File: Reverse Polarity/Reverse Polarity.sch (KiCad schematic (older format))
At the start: 16 parts, among them P1 CONN_01X04, P2 CONN_01X04, P3 CONN_01X04, P4 CONN_01X04, P5 CONN_01X04, P6 CONN_01X04, P7 CONN_01X04, P8 CONN_01X04

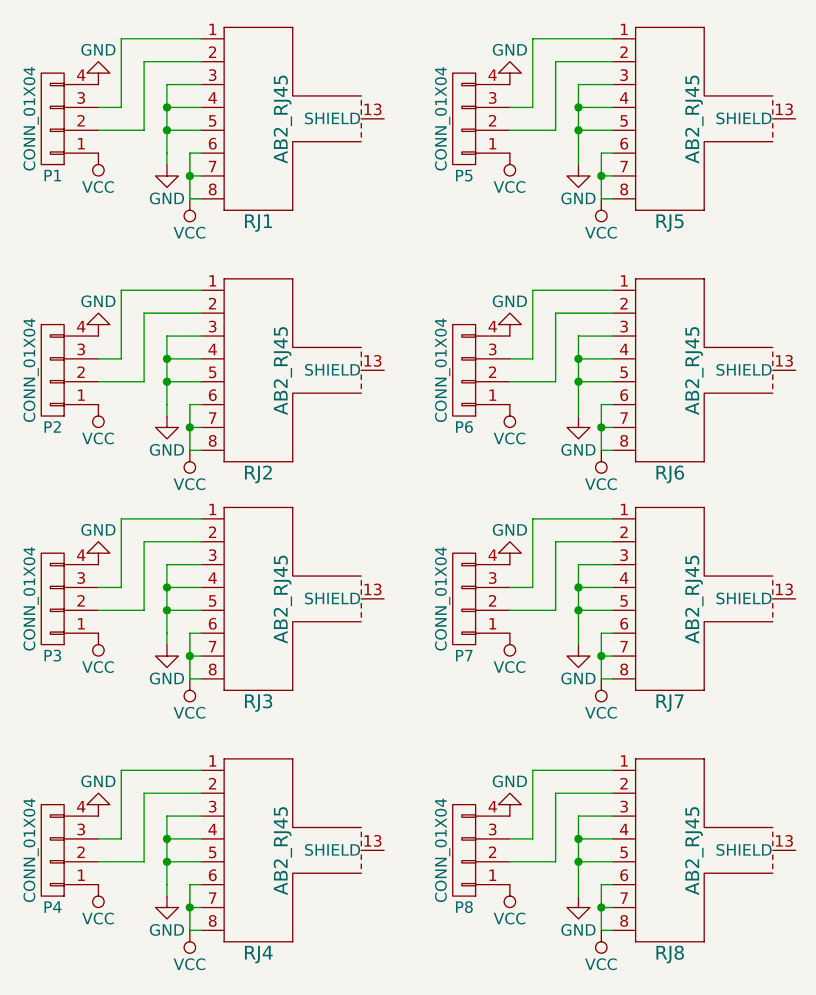
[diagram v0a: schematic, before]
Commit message: Also update schematic
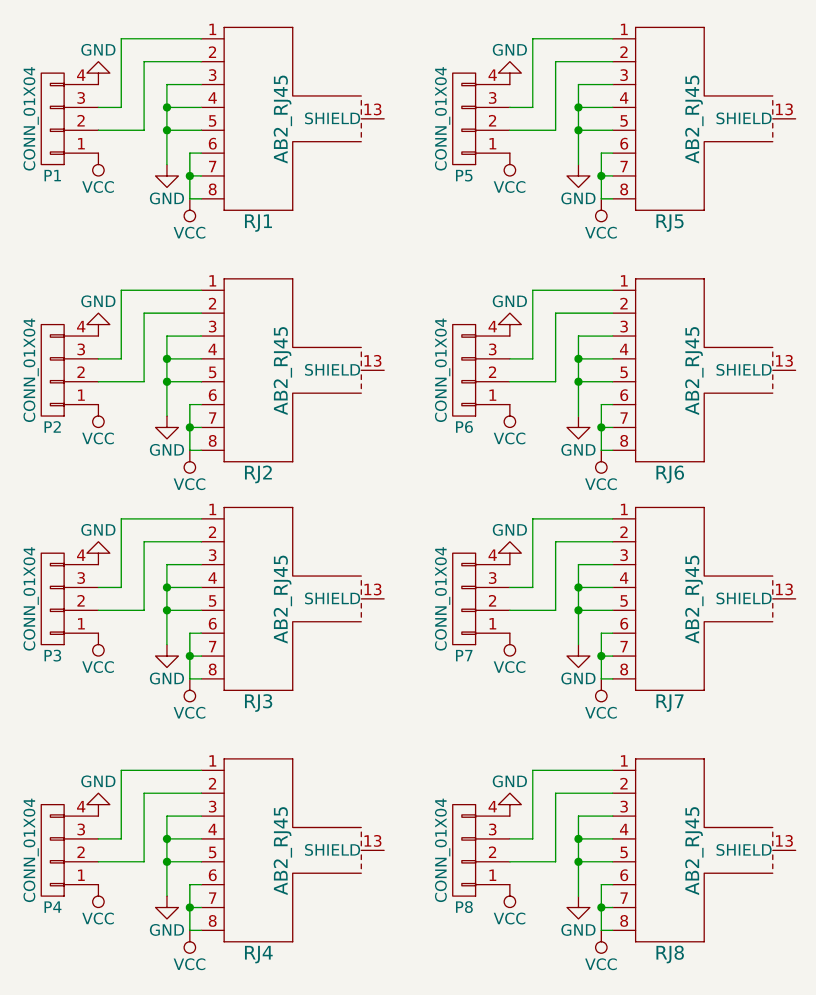
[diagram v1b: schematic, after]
